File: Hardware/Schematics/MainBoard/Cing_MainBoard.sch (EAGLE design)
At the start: 186 parts, among them IC1 L293D, IC2 LM2576S, IC3 FT232RL, IC4 BMP280, IC5 BME280, Q1 16mhz, Q2 BSS138, Q3 BSS138, Q4 BSS138, Q5 BSS138, Q6 NP2301AMR-G, Q7 NP2301AMR-G, T1 FS8205, T2 FS8205, U3 MPU-6050MPU6050, U4 CH330N

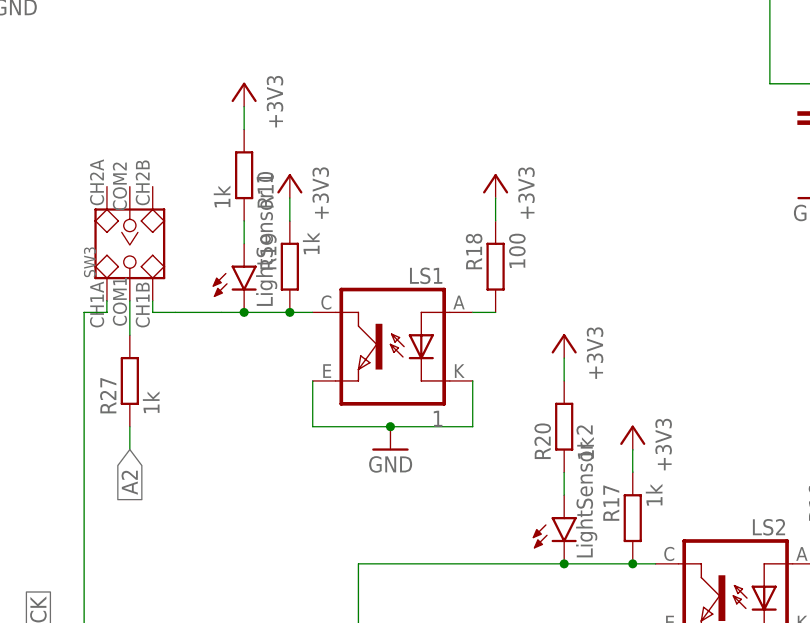
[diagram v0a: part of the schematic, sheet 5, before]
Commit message: fixing some bugs
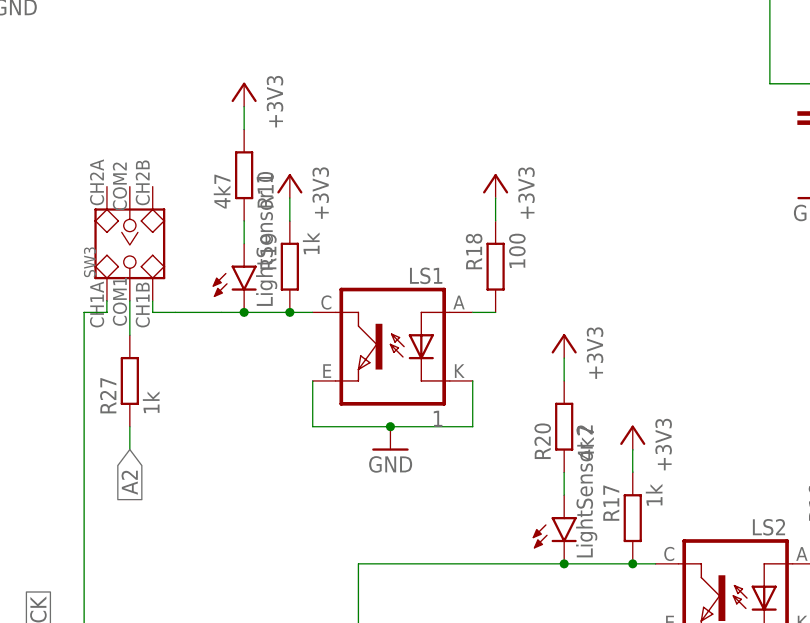
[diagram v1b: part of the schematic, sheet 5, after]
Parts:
- R10, R20: value 1k -> 4k7
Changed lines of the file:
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@@
 <part name="TXD2" library="led" library_urn="urn:adsk.eagle:library:259" deviceset="LED" device="SMT1206" package3d_urn="urn:adsk.eagle:package:15796/2" value="LightSensor 2"/>
 <part name="+3V17" library="supply1" library_urn="urn:adsk.eagle:library:371" deviceset="+3V3" device=""/>
-<part name="R10" library="rcl" library_urn="urn:adsk.eagle:library:334" deviceset="R-EU_" device="R1206" package3d_urn="urn:adsk.eagle:package:23540/2" override_package3d_urn="urn:adsk.eagle:package:11835284/2" override_package_urn="urn:adsk.eagle:footprint:23047/1" value="1k"/>
-<part name="R20" library="rcl" library_urn="urn:adsk.eagle:library:334" deviceset="R-EU_" device="R1206" package3d_urn="urn:adsk.eagle:package:23540/2" override_package3d_urn="urn:adsk.eagle:package:11835283/2" override_package_urn="urn:adsk.eagle:footprint:23047/1" value="1k"/>
+<part name="R10" library="rcl" library_urn="urn:adsk.eagle:library:334" deviceset="R-EU_" device="R1206" package3d_urn="urn:adsk.eagle:package:23540/2" override_package3d_urn="urn:adsk.eagle:package:11835284/2" override_package_urn="urn:adsk.eagle:footprint:23047/1" value="4k7"/>
+<part name="R20" library="rcl" library_urn="urn:adsk.eagle:library:334" deviceset="R-EU_" device="R1206" package3d_urn="urn:adsk.eagle:package:23540/2" override_package3d_urn="urn:adsk.eagle:package:11835283/2" override_package_urn="urn:adsk.eagle:footprint:23047/1" value="4k7"/>
 <part name="+3V18" library="supply1" library_urn="urn:adsk.eagle:library:371" deviceset="+3V3" device=""/>
 <part name="C5" library="rcl" library_urn="urn:adsk.eagle:library:334" deviceset="C-EU" device="C1206" package3d_urn="urn:adsk.eagle:package:23618/2" value="100n"/>
